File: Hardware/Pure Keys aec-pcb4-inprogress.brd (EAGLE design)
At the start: 99.7 x 66.4 mm, 72 parts, among them Q2 20MHz, U1 ATMEGA328P_TQFP

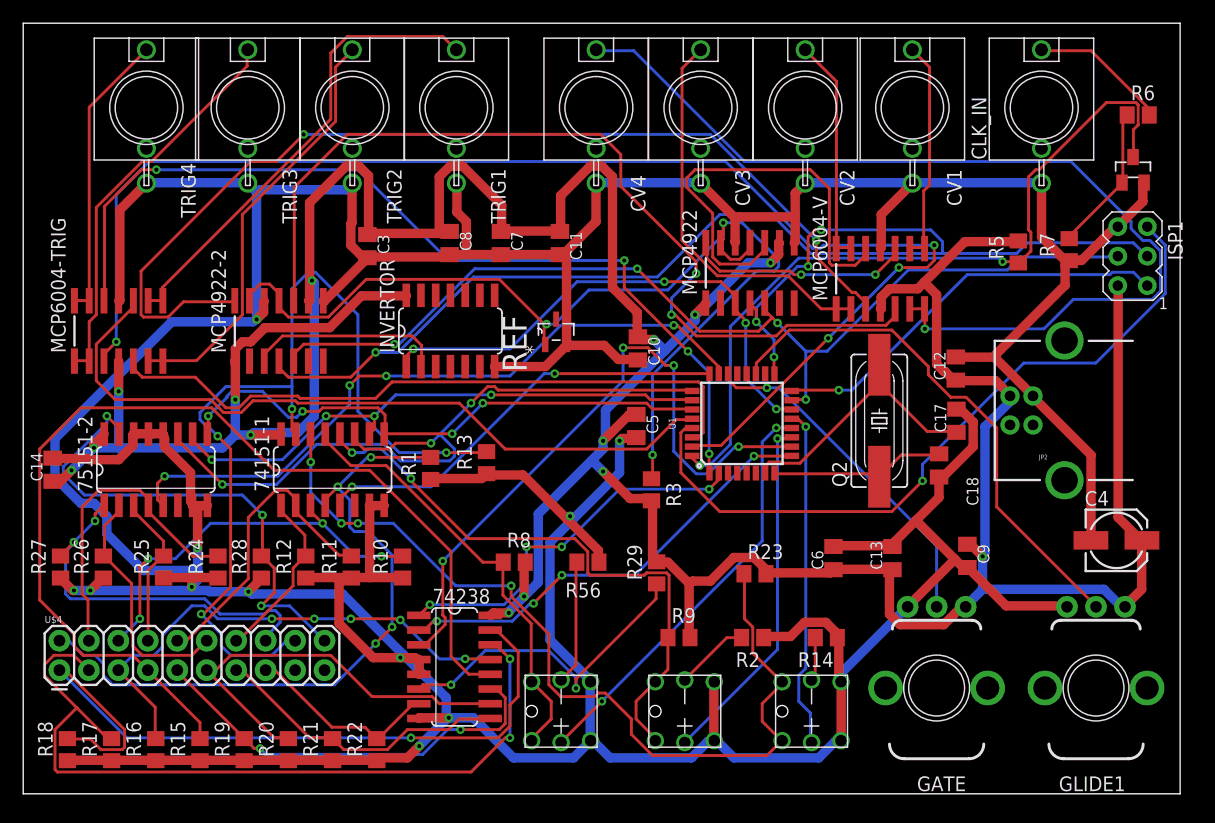
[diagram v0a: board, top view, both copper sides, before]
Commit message: tried new board layout
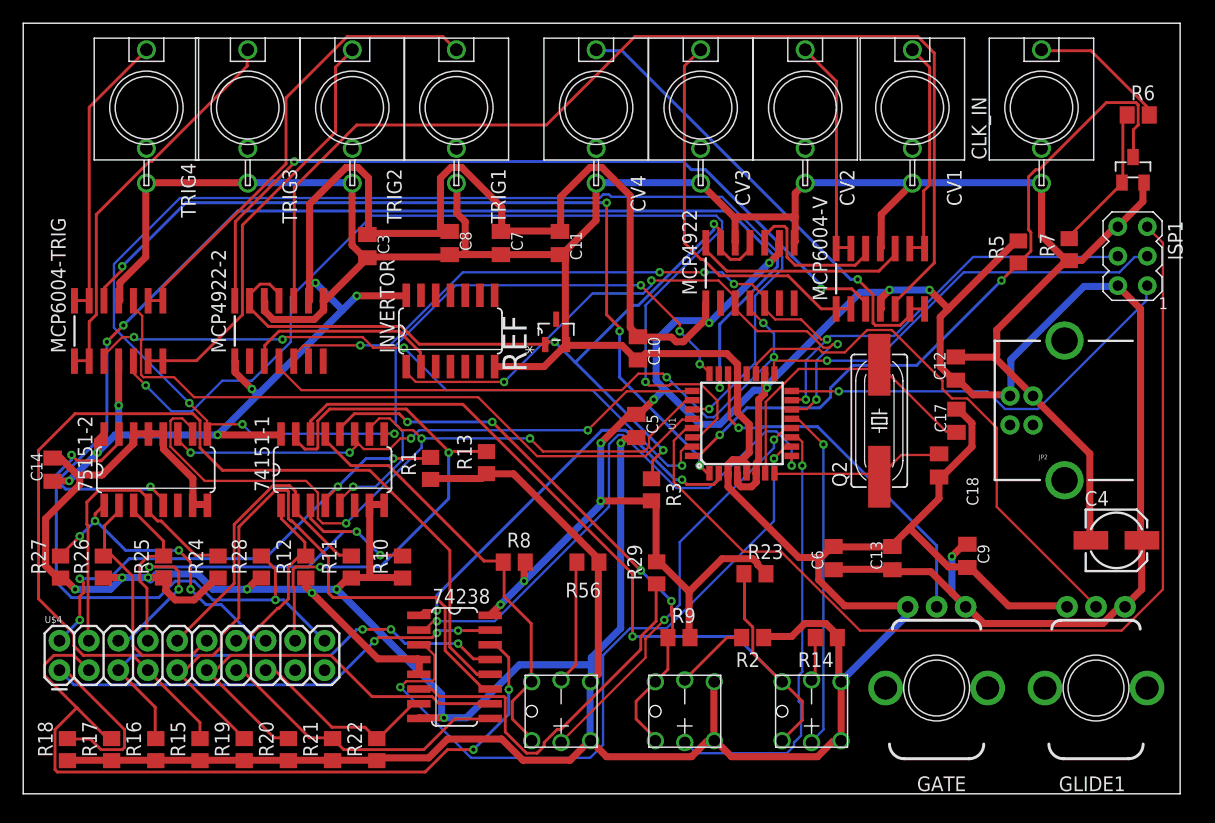
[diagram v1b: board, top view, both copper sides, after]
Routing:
- net A2IN: track 48.8 -> 115.7 mm
- net TRIG3: track 118.6 -> 58.1 mm
- net N$25: track 84.3 -> 40.5 mm
- net DBIN: track 59.1 -> 102.6 mm
- net TRIG2: track 57.5 -> 90.5 mm, vias 0 -> 2
- net MK4: track 80.7 -> 47.8 mm, vias 4 -> 2
- net VOUTB: track 37.4 -> 13.4 mm
- net RST: track 62.8 -> 86.4 mm, vias 1 -> 0
- net T4: track 36.4 -> 59.7 mm, vias 2 -> 0
- net SCK: track 113.7 -> 91.2 mm, vias 5 -> 4
- net VOUTC: track 87.3 -> 69.2 mm
- net A1IN: track 48.5 -> 66.4 mm, vias 4 -> 3
- net GND: track 558.0 -> 575.7 mm, vias 11 -> 8
- net 3VREF: track 89.4 -> 72.3 mm
- net MK0: track 58.8 -> 43.0 mm
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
